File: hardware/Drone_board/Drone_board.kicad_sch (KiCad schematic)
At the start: 12 parts, among them J1 Conn_01x08_Pin, J2 Conn_01x03_Pin, J3 Conn_01x03_Pin, J4 Conn_01x03_Pin, J5 Conn_01x03_Pin, J6 Conn_01x03_Pin, J7 Conn_01x03_Pin, U1 NUCLEO-L432KC, U3 NRF24L01_Breakout

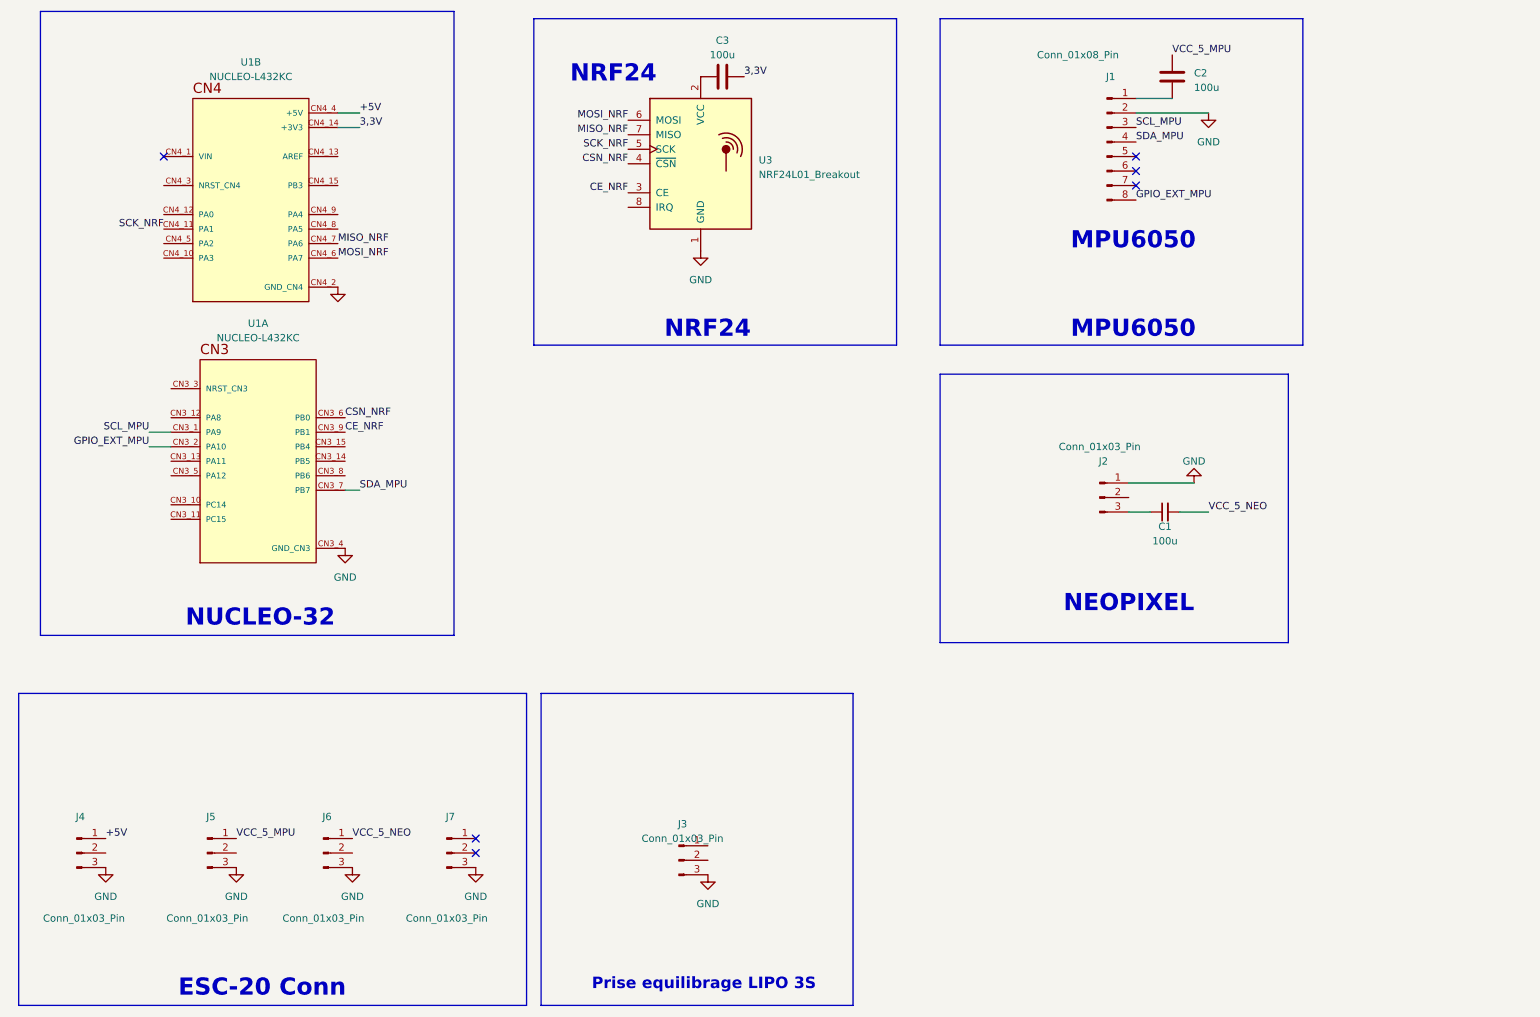
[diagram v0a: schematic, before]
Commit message: Schematic drone for validation
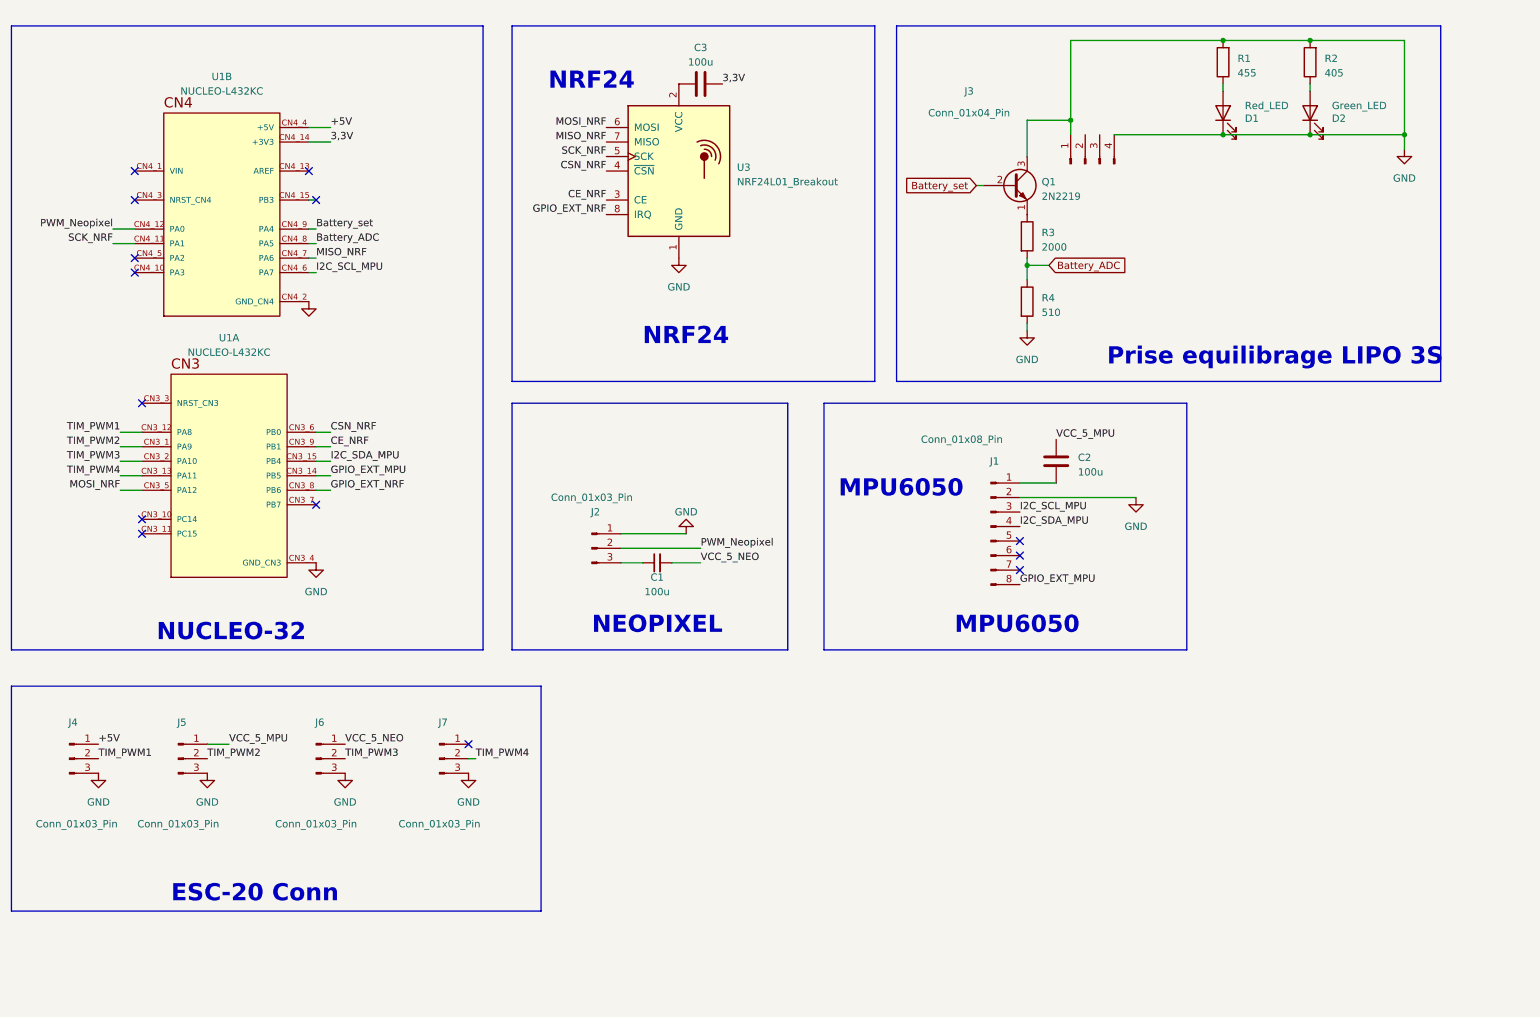
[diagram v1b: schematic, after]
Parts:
- removed J3: Conn_01x03_Pin, symbol Connector:Conn_01x03_Pin
- added D1: Red_LED, symbol Device:LED
- added D2: Green_LED, symbol Device:LED
- added J3: Conn_01x04_Pin, symbol Connector:Conn_01x04_Pin
- added Q1: 2N2219, Package_TO_SOT_THT:TO-39-3, symbol Transistor_BJT:2N2219
- added R1: 455, symbol Device:R
- added R2: 405, symbol Device:R
- added R3: 2000, symbol Device:R
- added R4: 510, symbol Device:R
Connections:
- net GND: now also D1.1 (K), D2.1 (K), J3.1 (Pin_1), J3.4 (Pin_4), Q1.3 (C), R1.2, R2.2, R4.2
- net GPIO_EXT_MPU: now also U1.CN3_14 (PB5); no longer U1.CN3_2 (PA10)
- net MOSI_NRF: now also U1.CN3_5 (PA12); no longer U1.CN4_6 (PA7)
- net TIM_PWM1: now reaches J4.2 (Pin_2)
- net TIM_PWM1: now also U1.CN3_12 (PA8)
- net PWM_Neopixel: now reaches U1.CN4_12 (PA0)
- net PWM_Neopixel: now also J2.2 (Pin_2)
- net Battery_ADC: now reaches U1.CN4_8 (PA5)
- net Battery_ADC: now also R3.2, R4.1
- net Battery_set: now reaches U1.CN4_9 (PA4)
- net Battery_set: now also Q1.2 (B)
- net TIM_PWM4: now reaches J7.2 (Pin_2)
- net TIM_PWM4: now also U1.CN3_13 (PA11)
- net TIM_PWM3: now reaches J6.2 (Pin_2)
- net TIM_PWM3: now also U1.CN3_2 (PA10)
- net GPIO_EXT_NRF: now reaches U3.8 (IRQ)
- net GPIO_EXT_NRF: now also U1.CN3_8 (PB6)
- net I2C_SDA_MPU: now reaches U1.CN3_15 (PB4)
- net I2C_SDA_MPU: now also J1.4 (Pin_4)
- net TIM_PWM2: now reaches J5.2 (Pin_2)
- net TIM_PWM2: now also U1.CN3_1 (PA9)
- net SCL_MPU renamed I2C_SCL_MPU
- net I2C_SCL_MPU: now also U1.CN4_6 (PA7); no longer U1.CN3_1 (PA9)
- net SDA_MPU: no longer names the net of U1.CN3_7 (PB7)
- net SDA_MPU: no longer J1.4 (Pin_4)
- new net: Q1.1 (E), R3.1
- new net: D2.2 (A), R2.1
- new net: D1.2 (A), R1.1
- no-connect marks 6 -> 14
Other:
- moved on the sheet: C1, C2, C3, J1, J2, J4, J5, J6, J7, U1A, U1B, U3
